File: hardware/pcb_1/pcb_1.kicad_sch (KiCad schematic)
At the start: 5 parts, among them J1 Connector, USB-TYPE-C-16P

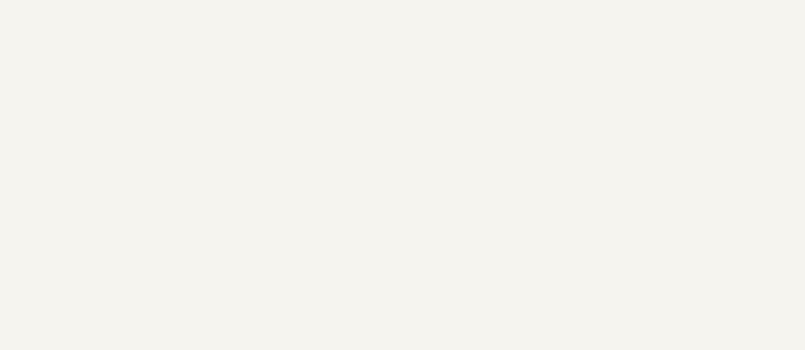
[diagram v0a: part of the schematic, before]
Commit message: test-workflow
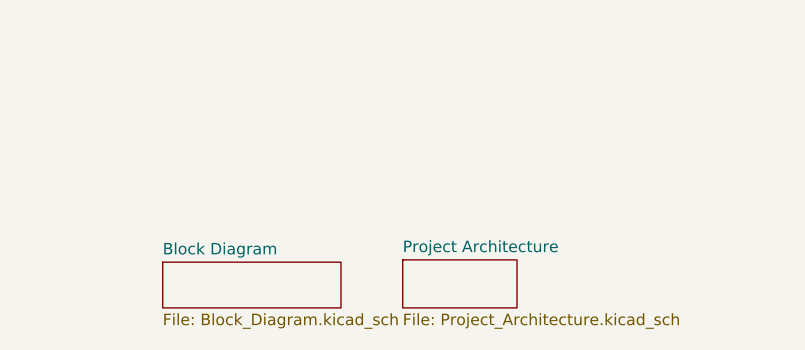
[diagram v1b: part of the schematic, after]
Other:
- added sheet Block Diagram (Block_Diagram.kicad_sch)
- added sheet Project Architecture (Project_Architecture.kicad_sch)
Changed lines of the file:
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@@
+		)
+	)
+	(sheet
+		(at 139.7 187.96)
+		(size 12.7 5.334)
+		(exclude_from_sim no)
+		(in_bom yes)
+		(on_board yes)
+		(dnp no)
+		(fields_autoplaced yes)
+		(stroke
+			(width 0.1524)
+			(type solid)
+		)
+		(fill
+			(color 0 0 0 0.0000)
+		)
+		(property "Sheetname" "Project Architecture"
+			(at 139.7 187.2484 0)
+			(effects
+				(font
+					(size 1.27 1.27)
+				)
+				(justify left bottom)
+			)
+		)
+		(property "Sheetfile" "Project_Architecture.kicad_sch"
+			(at 139.7 193.8786 0)
+			(effects
+				(font
+					(size 1.27 1.27)
+				)
+				(justify left top)
+			)
+		)
+		(instances
+			(project "pcb_1"
+				(path "/fa760f25-0aab-4539-8232-50b99fee633f"
+					(page "3")
+				)
+			)
+		)
+	)
+	(sheet
+		(at 113.03 188.214)
+		(size 19.812 5.08)
+		(exclude_from_sim no)
+		(in_bom yes)
+		(on_board yes)
+		(dnp no)
+		(fields_autoplaced yes)
+		(stroke
+			(width 0.1524)
+			(type solid)
+		)
+		(fill
+			(color 0 0 0 0.0000)
+		)
+		(property "Sheetname" "Block Diagram"
+			(at 113.03 187.5024 0)
+			(effects
+				(font
+					(size 1.27 1.27)
+				)
+				(justify left bottom)
+			)
+		)
+		(property "Sheetfile" "Block_Diagram.kicad_sch"
+			(at 113.03 193.8786 0)
+			(effects
+				(font
+					(size 1.27 1.27)
+				)
+				(justify left top)
+			)
+		)
+		(instances
+			(project "pcb_1"
+				(path "/fa760f25-0aab-4539-8232-50b99fee633f"
+					(page "2")
+				)
+			)
 		)
 	)

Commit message: Revert "test-workflow"
This reverts commit 1e65093ea42dd0d6fb7e03bbed3175e72afe33ec.
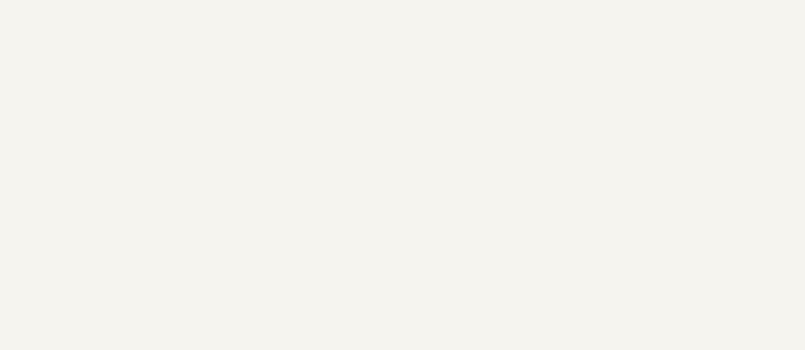
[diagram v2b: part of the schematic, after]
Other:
- removed sheet Block Diagram
- removed sheet Project Architecture
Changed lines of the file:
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@@
-		)
-	)
-	(sheet
-		(at 139.7 187.96)
-		(size 12.7 5.334)
-		(exclude_from_sim no)
-		(in_bom yes)
-		(on_board yes)
-		(dnp no)
-		(fields_autoplaced yes)
-		(stroke
-			(width 0.1524)
-			(type solid)
-		)
-		(fill
-			(color 0 0 0 0.0000)
-		)
-		(property "Sheetname" "Project Architecture"
-			(at 139.7 187.2484 0)
-			(effects
-				(font
-					(size 1.27 1.27)
-				)
-				(justify left bottom)
-			)
-		)
-		(property "Sheetfile" "Project_Architecture.kicad_sch"
-			(at 139.7 193.8786 0)
-			(effects
-				(font
-					(size 1.27 1.27)
-				)
-				(justify left top)
-			)
-		)
-		(instances
-			(project "pcb_1"
-				(path "/fa760f25-0aab-4539-8232-50b99fee633f"
-					(page "3")
-				)
-			)
-		)
-	)
-	(sheet
-		(at 113.03 188.214)
-		(size 19.812 5.08)
-		(exclude_from_sim no)
-		(in_bom yes)
-		(on_board yes)
-		(dnp no)
-		(fields_autoplaced yes)
-		(stroke
-			(width 0.1524)
-			(type solid)
-		)
-		(fill
-			(color 0 0 0 0.0000)
-		)
-		(property "Sheetname" "Block Diagram"
-			(at 113.03 187.5024 0)
-			(effects
-				(font
-					(size 1.27 1.27)
-				)
-				(justify left bottom)
-			)
-		)
-		(property "Sheetfile" "Block_Diagram.kicad_sch"
-			(at 113.03 193.8786 0)
-			(effects
-				(font
-					(size 1.27 1.27)
-				)
-				(justify left top)
-			)
-		)
-		(instances
-			(project "pcb_1"
-				(path "/fa760f25-0aab-4539-8232-50b99fee633f"
-					(page "2")
-				)
-			)
 		)
 	)
